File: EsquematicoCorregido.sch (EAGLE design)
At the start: 25 parts, among them IC1 OPA991TIDCKR, IC2 AD8226ARZ-RL, IC3 OPA991TIDCKR, IC4 ESP32-S3-WROOM-1-N16R8, IC5 OPA991TIDCKR, IC6 MAX30102EFD+T, IC7 LP38692MP-3.3_NOPB, IC8 LP38692MP-1.8_NOPB, IC9 REF2033AIDDCT

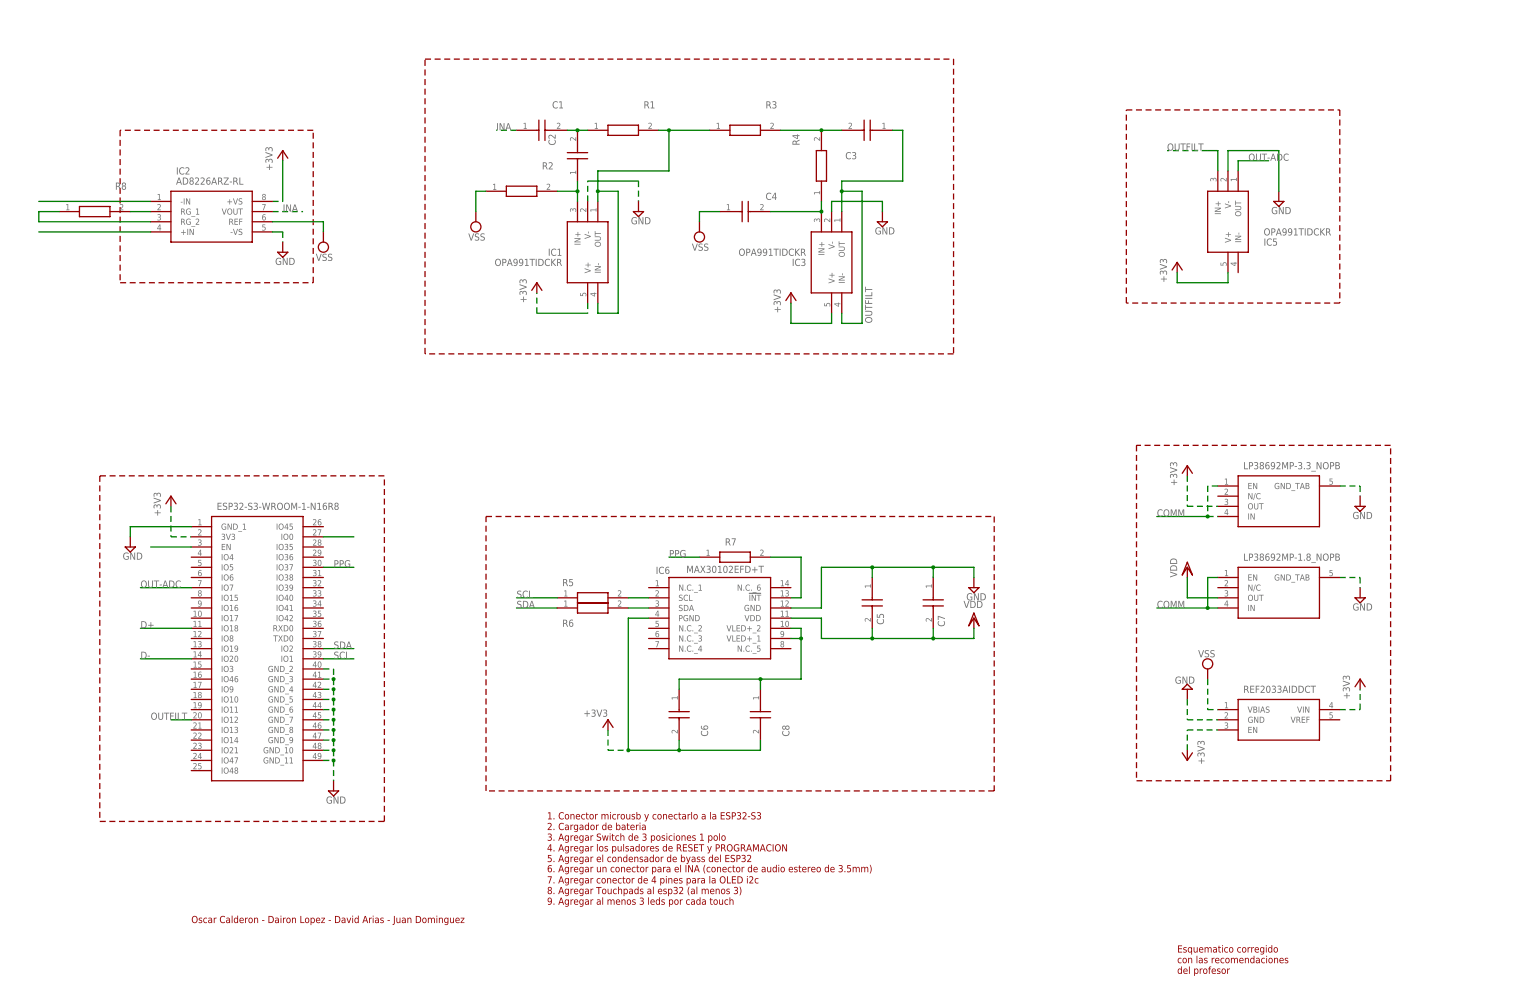
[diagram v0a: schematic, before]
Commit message: ultima actualización, correcion de los puntos
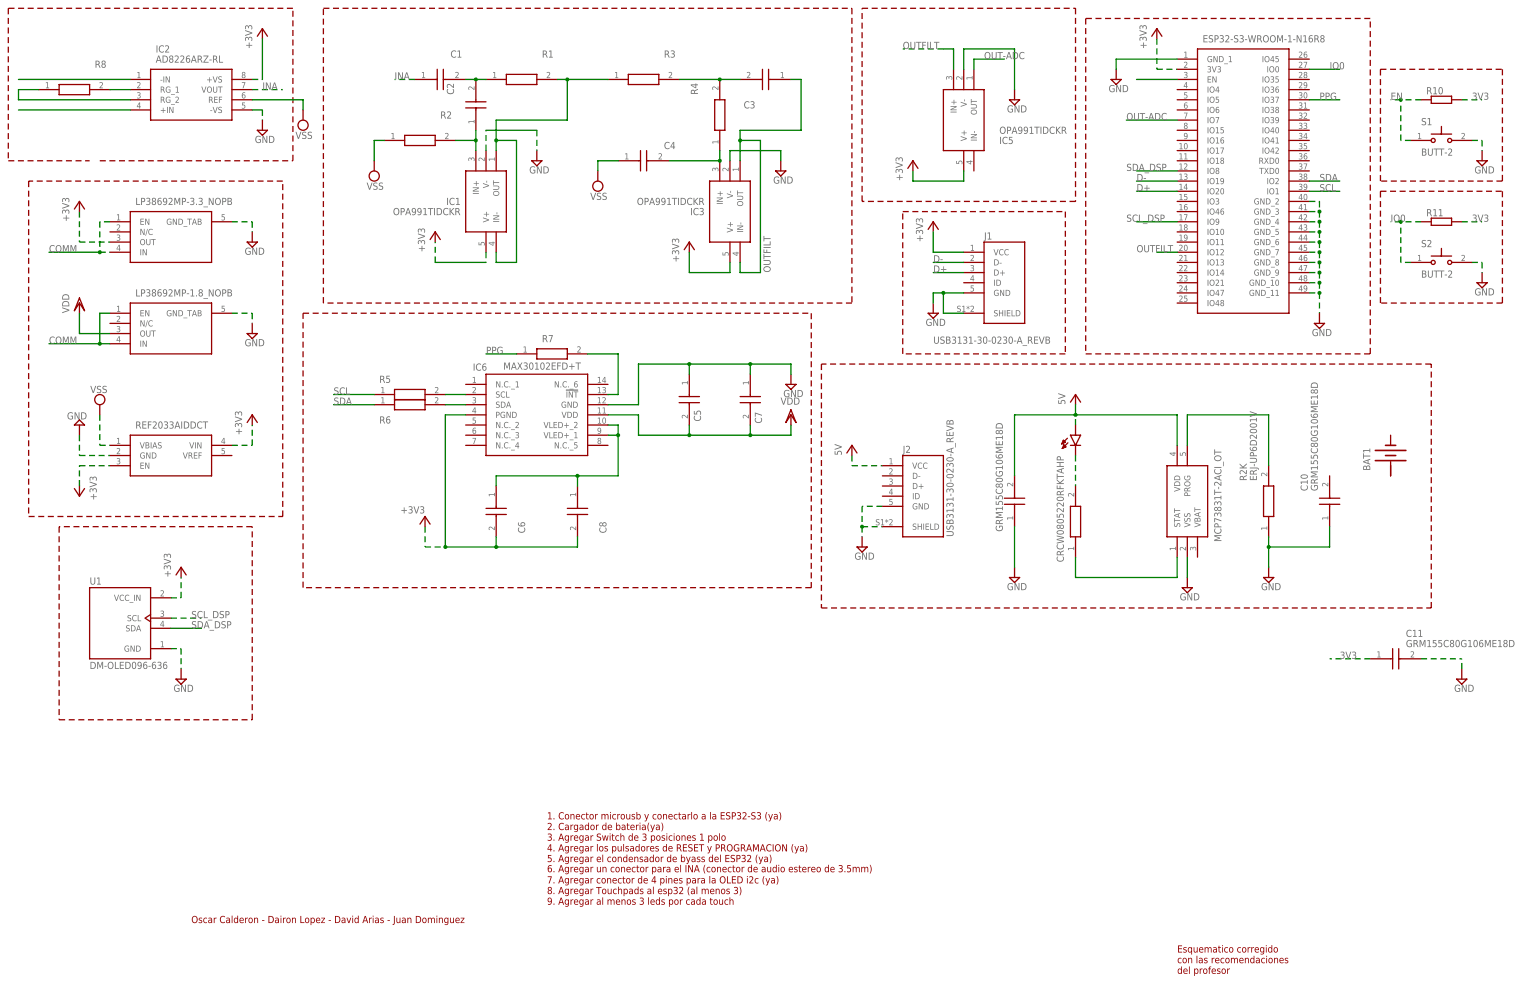
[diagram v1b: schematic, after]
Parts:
- added BAT1: (no value), special:BATTERY
- added C10, C11, C9: GRM155C80G106ME18D, GRM155C80G106ME18D:GRM155C80G106ME18D
- added D1: HLMP6, display-hp:HLMP6
- added IC10: MCP73831T-2ACI_OT, MCP73831T-2ACI_OT:MCP73831T-2ACI_OT
- added J1, J2: USB3131-30-0230-A_REVB, USB3131-30-0230-A_REVB:USB3131-30-0230-A_REVB
- added R10, R11: (no value), resistor-shunt:BVS
- added R2K: ERJ-UP6D2001V, ERJ-UP6D2001V:ERJ-UP6D2001V
- added R9: CRCW0805220RFKTAHP, CRCW0805220RFKTAHP:CRCW0805220RFKTAHP
- added S1, S2: BUTT-2, BUTT-2:BUTT-2
- added U1: DM-OLED096-636, DM-OLED096-636:DM-OLED096-636
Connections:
- removed net N$5: IC4.IO0
- new net 3V3: C11.1, R10.1, R11.1
- new net 5V: C9.2, D1.A, IC10.VDD, J2.VCC
- new net EN: R10.2, S1.1
- new net IO0: IC4.IO0, R11.2, S2.1
- new net N$16: D1.K, R9.2
- new net N$17: IC10.PROG, R2K.2
- new net N$18: IC10.STAT, R9.1
- new net SCL_DSP: IC4.IO9, U1.SCL
- new net SDA_DSP: IC4.IO8, U1.SDA
- net +3V3: now also J1.VCC, U1.VCC_IN
- net D+: now also IC4.IO20, J1.D+; no longer IC4.IO18
- net D-: now also IC4.IO19, J1.D-; no longer IC4.IO20
- net GND: now also C10.1, C11.2, C9.1, IC10.VSS, J1.GND, J1.SHIELD, J2.GND, J2.SHIELD, R2K.1, S1.2, S2.2, U1.GND
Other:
- note added: "1. Conector microusb y conectarlo a la ESP32-S3 (ya) 2. Cargador de bateria(ya) 3. Agregar Switch de 3 posiciones 1 polo 4. Agregar los pulsadores de RESET y PROGRAMACION (ya) 5. Agregar el condensador de byass del ESP32 (ya)"
- note added: "7. Agregar conector de 4 pines para la OLED i2c (ya) 8. Agregar Touchpads al esp32 (al menos 3) 9. Agregar al menos 3 leds por cada touch"
- note removed: "1. Conector microusb y conectarlo a la ESP32-S3 2. Cargador de bateria 3. Agregar Switch de 3 posiciones 1 polo 4. Agregar los pulsadores de RESET y PROGRAMACION 5. Agregar el condensador de byass del ESP32"
- note removed: "7. Agregar conector de 4 pines para la OLED i2c 8. Agregar Touchpads al esp32 (al menos 3) 9. Agregar al menos 3 leds por cada touch"
- moved on the sheet: C1, C2, C3, C4, C5, C6, C7, C8, IC1, IC2, IC3, IC5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
